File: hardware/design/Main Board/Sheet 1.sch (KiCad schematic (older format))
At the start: 1 part

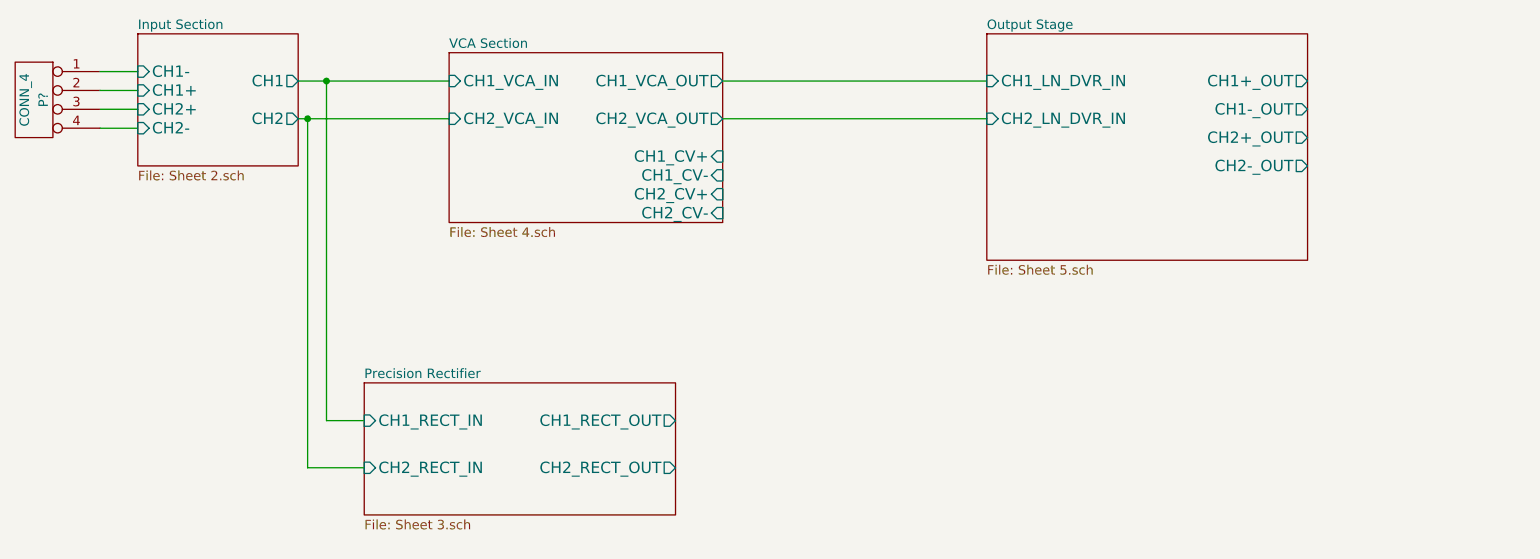
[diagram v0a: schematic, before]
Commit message: Op Amp Changes
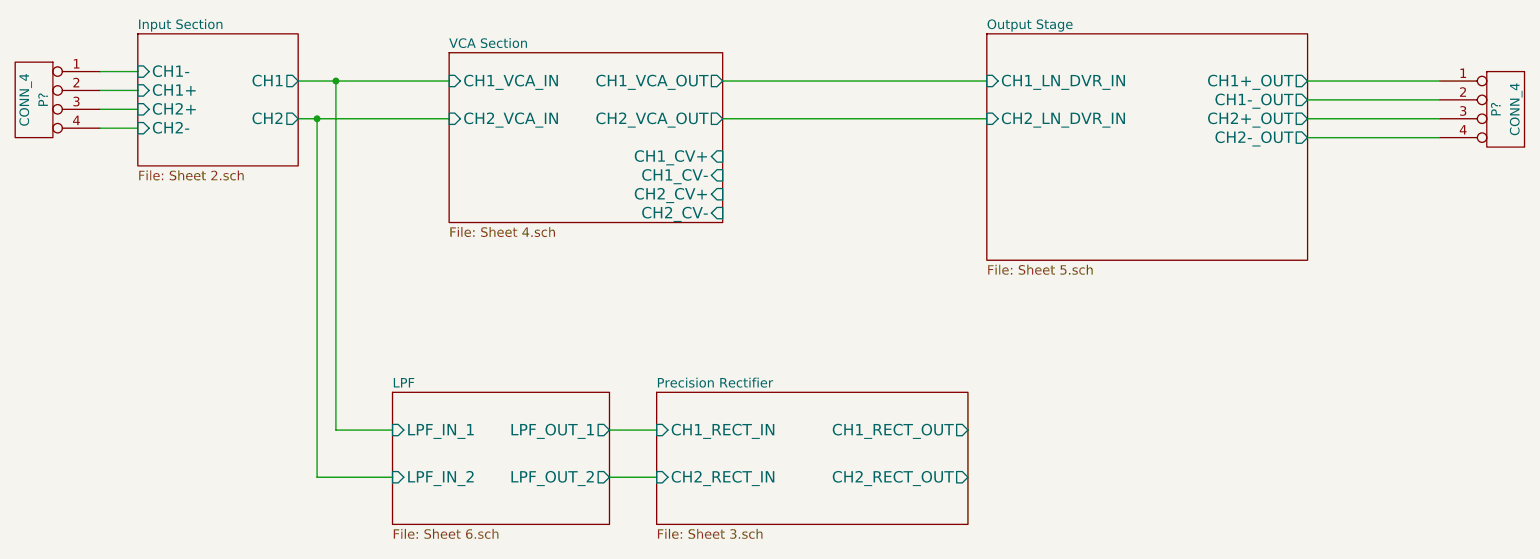
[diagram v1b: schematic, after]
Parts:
- added P?: CONN_4, symbol CONN_4
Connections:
- net Output Stage/CH1+_OUT: now also P?.1 (P1)
- net Output Stage/CH1-_OUT: now also P?.2 (P2)
- net Output Stage/CH2+_OUT: now also P?.3 (P3)
- net Output Stage/CH2-_OUT: now also P?.4 (P4)
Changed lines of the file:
@@
 $Descr A4 11693 8268
 encoding utf-8
-Sheet 1 5
+Sheet 1 6
 Title ""
-Date "29 apr 2014"
+Date "2 may 2014"
 Rev ""
 Comp ""
@@
 	1500 2750 1700 2750
 $Sheet
-S 2900 4100 1650 700
+S 4450 4150 1650 700
 U 534DCE54
 F0 "Precision Rectifier" 50
 F1 "Sheet 3.sch" 50
-F2 "CH1_RECT_IN" I L 2900 4300 60
-F3 "CH2_RECT_IN" I L 2900 4550 60
-F4 "CH1_RECT_OUT" O R 4550 4300 60
-F5 "CH2_RECT_OUT" O R 4550 4550 60
+F2 "CH1_RECT_IN" I L 4450 4350 60
+F3 "CH2_RECT_IN" I L 4450 4600 60
+F4 "CH1_RECT_OUT" O R 6100 4350 60
+F5 "CH2_RECT_OUT" O R 6100 4600 60
 $EndSheet
 Wire Wire Line
 	2550 2700 3350 2700
 Wire Wire Line
-	2600 2700 2600 4550
-Wire Wire Line
 	2550 2500 3350 2500
-Wire Wire Line
-	2700 2500 2700 4300
 $Sheet
 S 3350 2350 1450 900
@@
 F9 "CH2_CV+" I R 4800 3100 60
 $EndSheet
-Connection ~ 2700 2500
-Connection ~ 2600 2700
-Wire Wire Line
-	2700 4300 2900 4300
-Wire Wire Line
-	2600 4550 2900 4550
 $Sheet
 S 6200 2250 1700 1200
@@
 F2 "CH1_LN_DVR_IN" I L 6200 2500 60
 F3 "CH1+_OUT" O R 7900 2500 60
-F4 "CH1-_OUT" O R 7900 2650 60
+F4 "CH1-_OUT" O R 7900 2600 60
 F5 "CH2_LN_DVR_IN" I L 6200 2700 60
-F6 "CH2+_OUT" O R 7900 2800 60
-F7 "CH2-_OUT" O R 7900 2950 60
+F6 "CH2+_OUT" O R 7900 2700 60
+F7 "CH2-_OUT" O R 7900 2800 60
 $EndSheet
 Wire Wire Line
@@
 Wire Wire Line
 	4800 2700 6200 2700
+$Comp
+L CONN_4 P?
+U 1 1 5362E417
+P 8950 2650
+F 0 "P?" V 8900 2650 50  0000 C CNN
+F 1 "CONN_4" V 9000 2650 50  0000 C CNN
+F 2 "" H 8950 2650 60  0000 C CNN
+F 3 "" H 8950 2650 60  0000 C CNN
+	1    8950 2650
+	1    0    0    -1
+$EndComp
+$Sheet
+S 3050 4150 1150 700
+U 5362F285
+F0 "LPF" 50
+F1 "Sheet 6.sch" 50
+F2 "LPF_IN_1" I L 3050 4350 60
+F3 "LPF_IN_2" I L 3050 4600 60
+F4 "LPF_OUT_1" O R 4200 4350 60
+F5 "LPF_OUT_2" O R 4200 4600 60
+$EndSheet
+Wire Wire Line
+	3050 4350 2750 4350
+Wire Wire Line
+	2750 4350 2750 2500
+Connection ~ 2750 2500
+Wire Wire Line
+	2650 2700 2650 4600
+Wire Wire Line
+	2650 4600 3050 4600
+Connection ~ 2650 2700
+Wire Wire Line
+	4200 4350 4450 4350
+Wire Wire Line
+	4200 4600 4450 4600
+Wire Wire Line
+	8600 2500 7900 2500
+Wire Wire Line
+	8600 2600 7900 2600
+Wire Wire Line
+	8600 2700 7900 2700
+Wire Wire Line
+	8600 2800 7900 2800
 $EndSCHEMATC
